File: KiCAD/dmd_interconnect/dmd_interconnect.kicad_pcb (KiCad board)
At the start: 2 copper layers, 7 x 5 mm, 1 part, among them U1 DLP301S

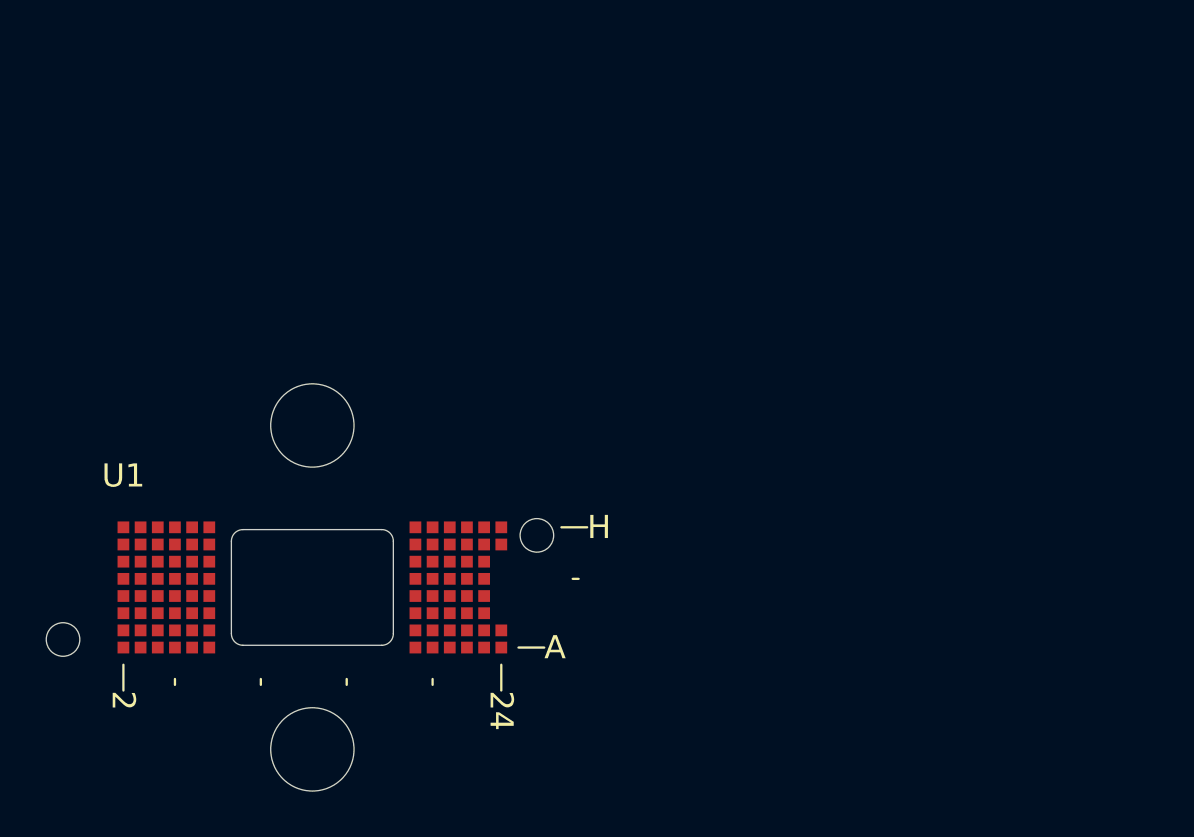
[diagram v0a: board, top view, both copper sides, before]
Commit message: dmd interconnect work 1st pass
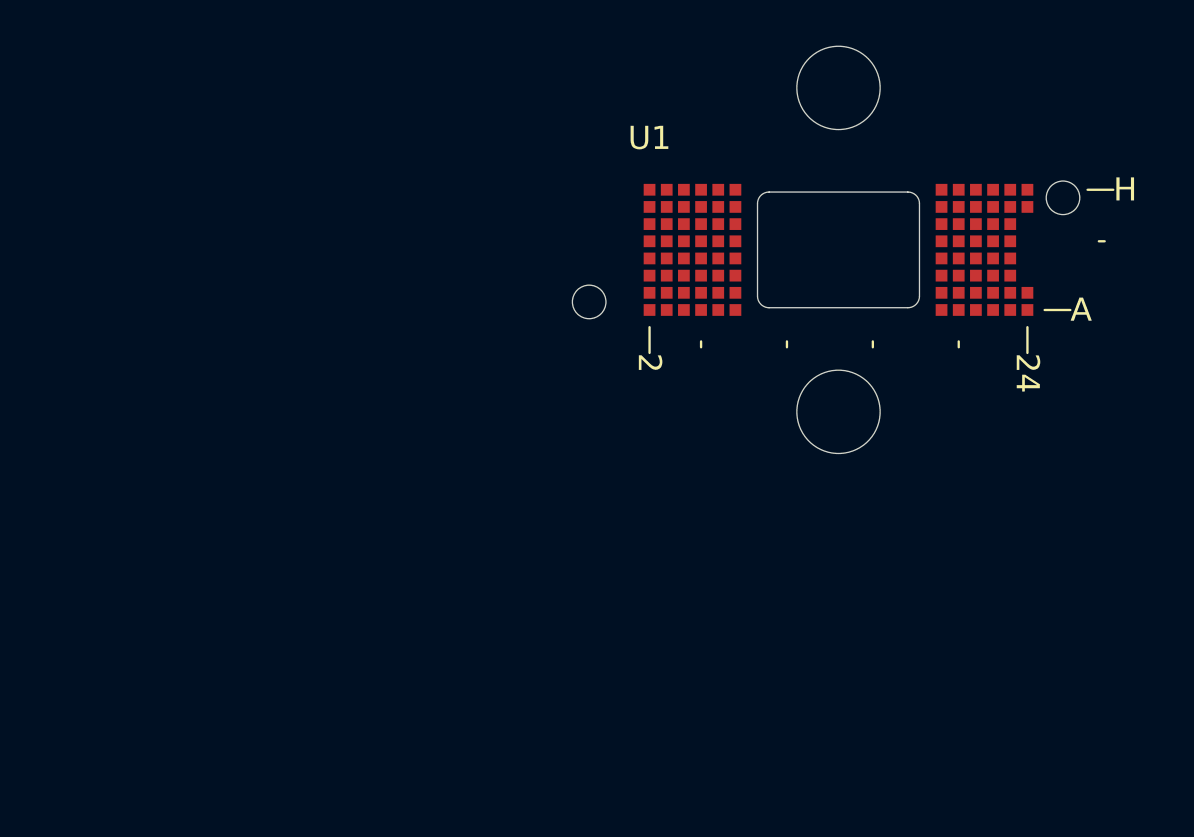
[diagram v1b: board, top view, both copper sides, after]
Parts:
- moved U1 27.0 mm to (173.3, 56.6)
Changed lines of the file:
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@@
 	(footprint "tp_library:LGA99_FQS"
 		(layer "F.Cu")
-		(at 150.5336 71.2016)
+		(at 173.2736 56.6116)
 		(tags "DLP3310AFQM ")
 		(property "Reference" "U1"
@@
 			(layer "F.CrtYd")
 		)
-		(fp_text user "2"
-			(at -8.1664 4.4544 270)
+		(fp_text user "A"
+			(at 10.0224 2.5984 0)
 			(unlocked yes)
 			(layer "F.SilkS")
@@
 			)
 		)
-		(fp_text user "A"
-			(at 10.0224 2.5984 0)
+		(fp_text user "2"
+			(at -8.1664 4.4544 270)
 			(unlocked yes)
 			(layer "F.SilkS")
@@
 			)
 		)
-		(fp_text user "H"
-			(at 11.8784 -2.5984 0)
+		(fp_text user "24"
+			(at 8.1664 4.4544 270)
 			(unlocked yes)
 			(layer "F.SilkS")
@@
 			)
 		)
-		(fp_text user "24"
-			(at 8.1664 4.4544 270)
+		(fp_text user "H"
+			(at 11.8784 -2.5984 0)
 			(unlocked yes)
 			(layer "F.SilkS")
@@
 		)
 		(embedded_fonts no)
-		(model "${KIPRJMOD}/custom_dlp.pretty/LGA99_FQS-customized.step"
+		(model "${KIPRJMOD}/../STEP/LGA99_FQS-customized.step"
 			(offset
 				(xyz -1.7424 0 5.5)
